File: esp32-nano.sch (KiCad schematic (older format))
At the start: 41 parts, among them K1 SW_MEC_5E, K2 SW_MEC_5E, P2 Conn_01x12, P3 Conn_01x18, U1 CP2102N-A01-GQFN28, U2 ME6211C33M5G, U3 MPU-6050, U4 ESP32PICO_D4, U5 OLED-12880

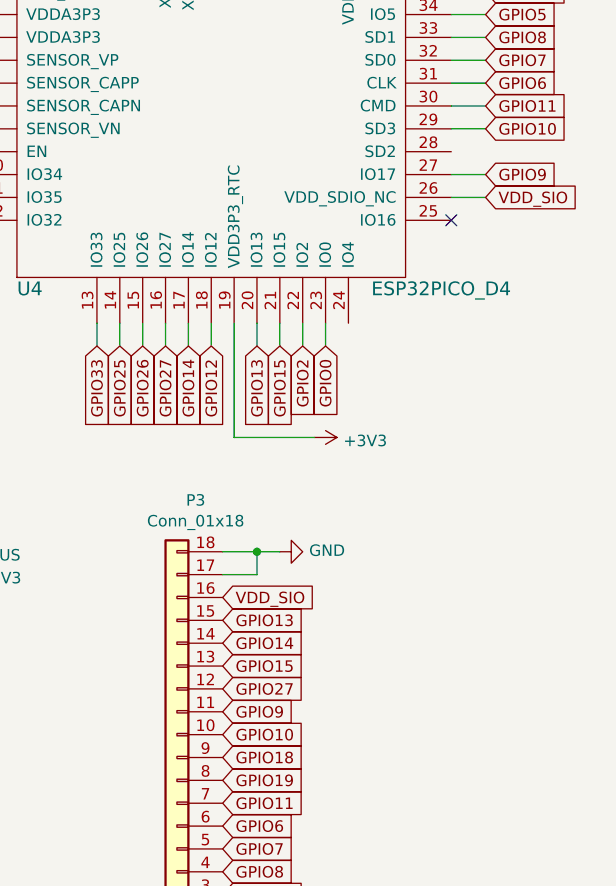
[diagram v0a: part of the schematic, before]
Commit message: .
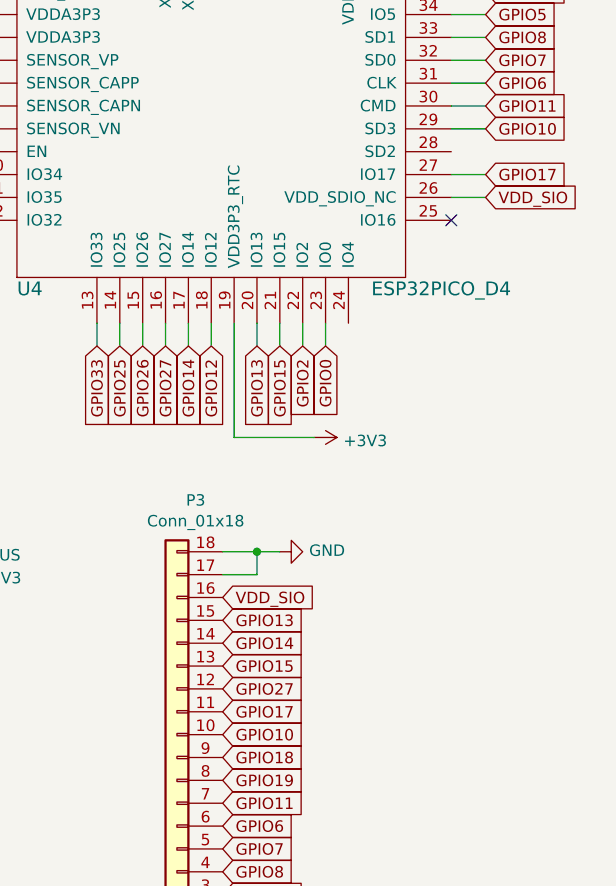
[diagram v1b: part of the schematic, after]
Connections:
- net GPIO9 renamed GPIO17
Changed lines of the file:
@@
 GPIO10
 Text GLabel 10350 2900 2    50   Input ~ 0
-GPIO9
+GPIO17
 Wire Wire Line
 	10200 2000 10350 2000
@@
 GPIO27
 Text GLabel 9200 5250 2    50   Input ~ 0
-GPIO9
+GPIO17
 Text GLabel 9200 5350 2    50   Input ~ 0
 GPIO10
